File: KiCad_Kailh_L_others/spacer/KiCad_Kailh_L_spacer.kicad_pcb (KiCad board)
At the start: 2 copper layers, 138.1 x 100 mm, 12 parts

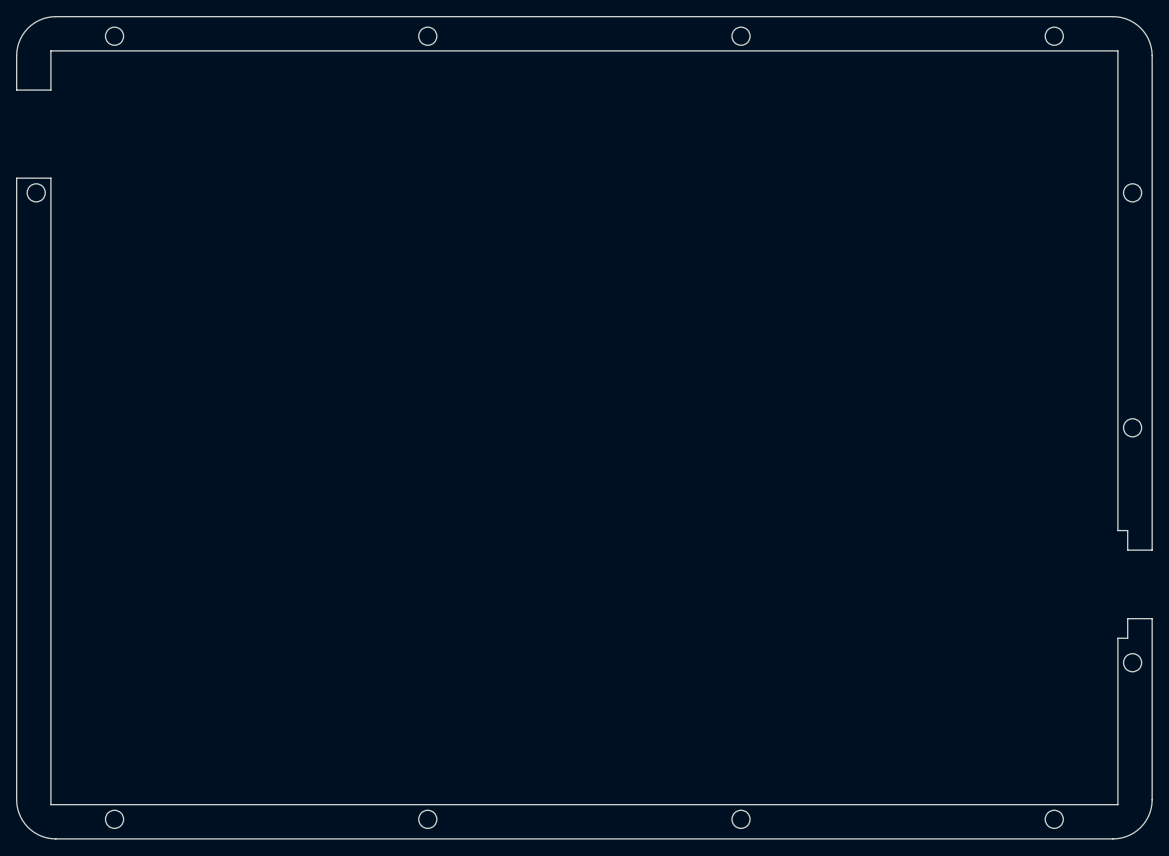
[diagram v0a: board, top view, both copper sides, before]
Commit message: feat: ガワがすべて完成
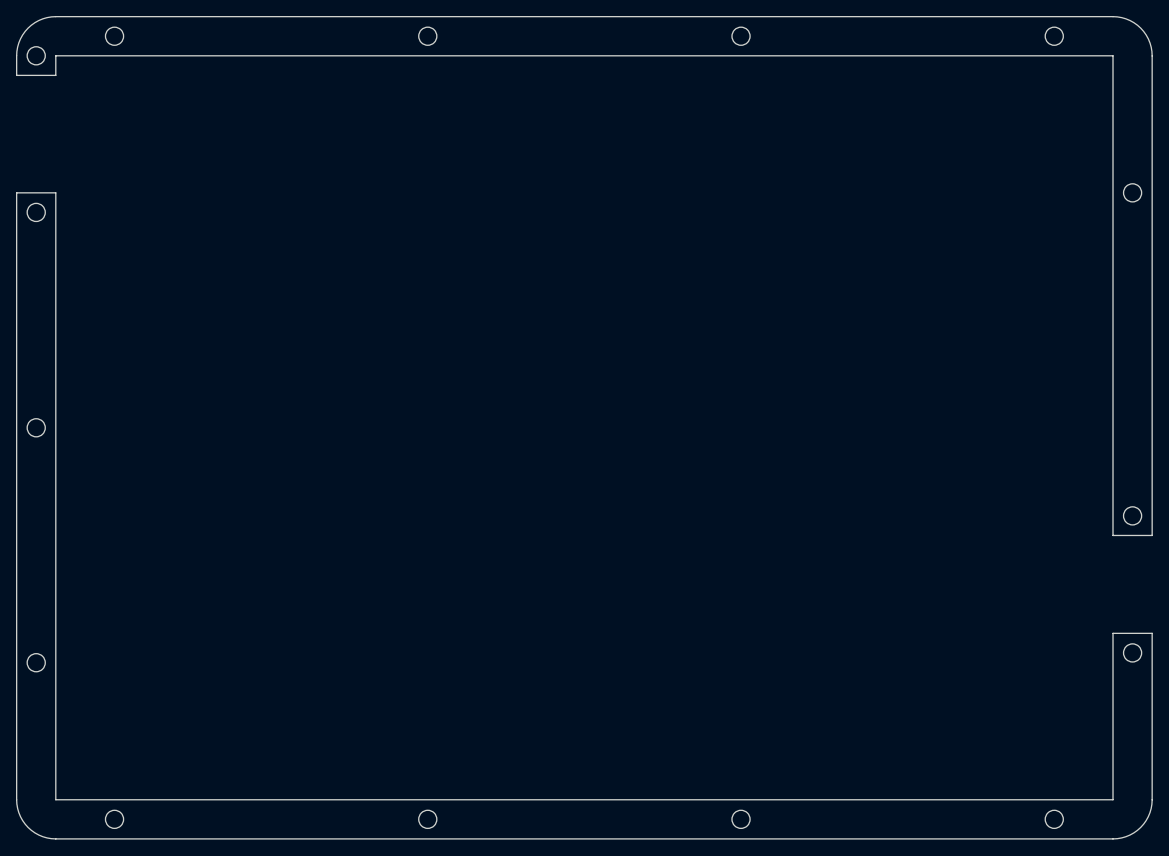
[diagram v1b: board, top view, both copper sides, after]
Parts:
- added H2: MountingHole_2.2mm_M2, MountingHole:MountingHole_2.2mm_M2, F.Cu at (83.3, 95.2)
- added H2: MountingHole_2.2mm_M2, MountingHole:MountingHole_2.2mm_M2, F.Cu at (83.3, 50.0)
- added H9: MountingHole_2.2mm_M2, MountingHole:MountingHole_2.2mm_M2, F.Cu at (83.3, 123.8)
- moved H2 10.7 mm to (216.7, 106.0)
- moved H7 2.38 mm to (83.3, 69.1)
- moved H14 1.19 mm to (216.7, 122.6)
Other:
- outline, holes or cut-outs redrawn
